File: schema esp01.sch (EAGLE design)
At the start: 8 parts

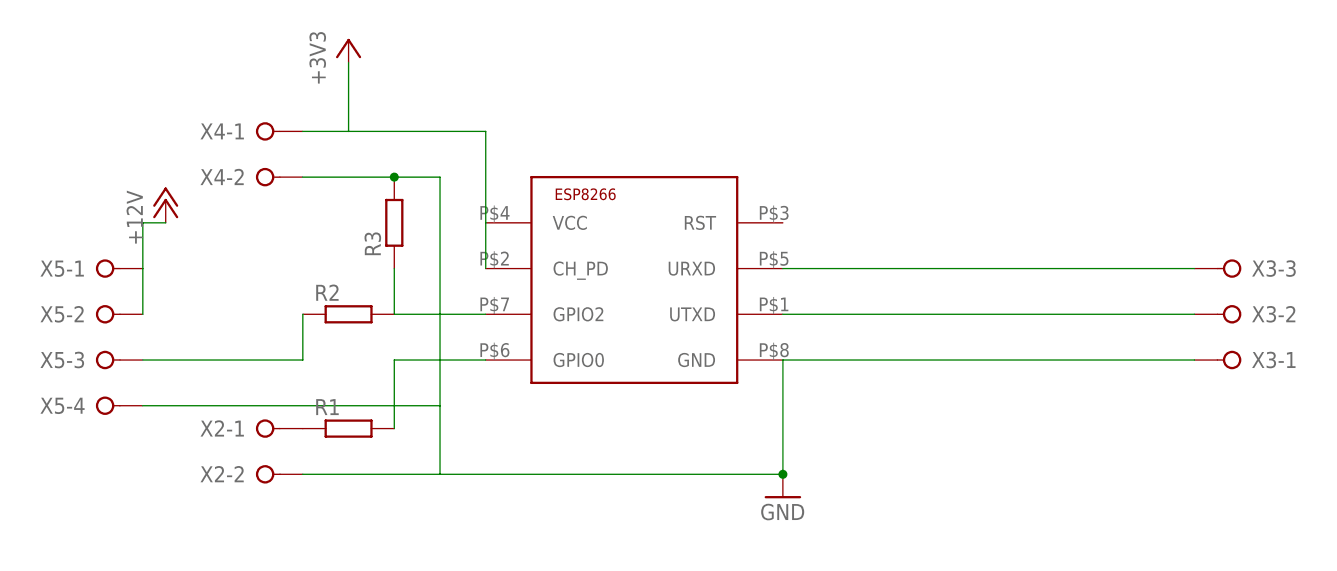
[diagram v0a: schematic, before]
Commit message: +
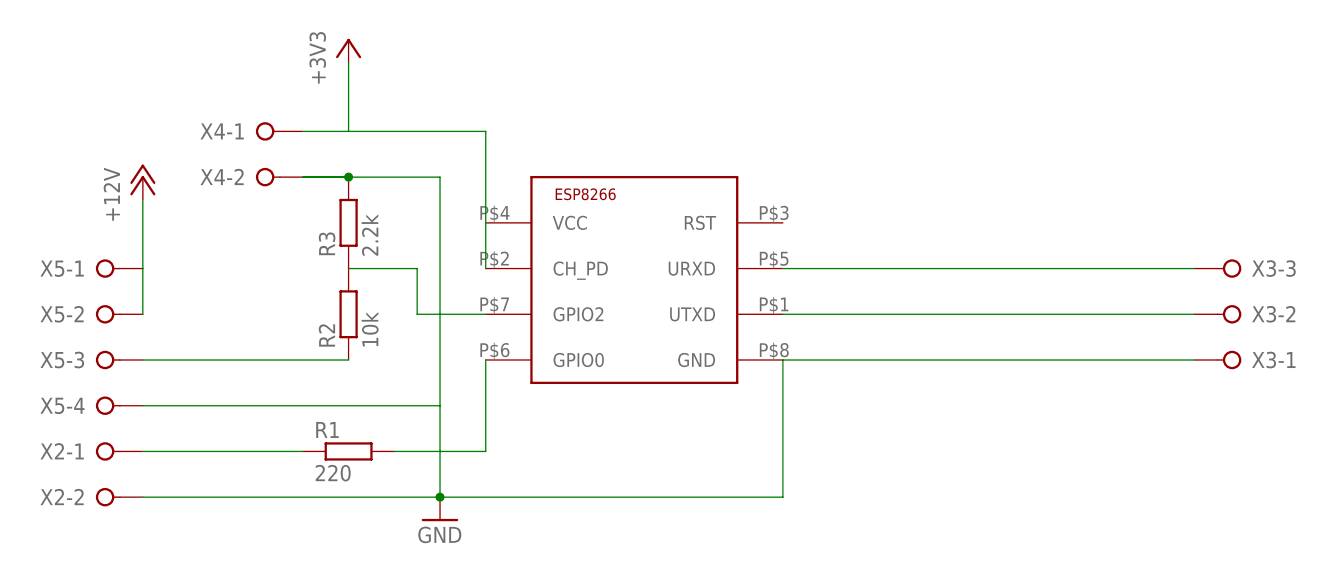
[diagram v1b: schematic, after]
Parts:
- R1: value (none) -> 220
- R2: value (none) -> 10k
- R3: value (none) -> 2.2k
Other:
- moved on the sheet: R1, R2, R3, X2-1, X2-2
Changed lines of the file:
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@@
 <part name="X2" library="con-wago-508" deviceset="W237-02P" device=""/>
 <part name="X3" library="con-wago-508" deviceset="W237-3E" device=""/>
-<part name="R1" library="rcl" deviceset="R-EU_" device="0204/7"/>
+<part name="R1" library="rcl" deviceset="R-EU_" device="0204/7" value="220"/>
 <part name="X4" library="con-wago-508" deviceset="W237-02P" device=""/>
 <part name="+3V1" library="supply1" deviceset="+3V3" device=""/>
-<part name="R2" library="rcl" deviceset="R-EU_" device="0204/7"/>
-<part name="R3" library="rcl" deviceset="R-EU_" device="0204/7"/>
+<part name="R2" library="rcl" deviceset="R-EU_" device="0204/7" value="10k"/>
+<part name="R3" library="rcl" deviceset="R-EU_" device="0204/7" value="2.2k"/>
 <part name="X5" library="con-wago-508" deviceset="W237-04P" device=""/>
 <part name="P+1" library="supply1" deviceset="+12V" device=""/>
@@
 <instances>
 <instance part="U$1" gate="G$1" x="12.7" y="68.58"/>
-<instance part="X2" gate="-1" x="-12.7" y="60.96"/>
-<instance part="X2" gate="-2" x="-12.7" y="55.88"/>
+<instance part="X2" gate="-1" x="-30.48" y="58.42"/>
+<instance part="X2" gate="-2" x="-30.48" y="53.34"/>
 <instance part="X3" gate="-1" x="96.52" y="68.58" rot="R180"/>
 <instance part="X3" gate="-2" x="96.52" y="73.66" rot="R180"/>
 <instance part="X3" gate="-3" x="96.52" y="78.74" rot="R180"/>
-<instance part="R1" gate="G$1" x="-2.54" y="60.96"/>
+<instance part="R1" gate="G$1" x="-2.54" y="58.42"/>
 <instance part="X4" gate="-1" x="-12.7" y="93.98"/>
 <instance part="X4" gate="-2" x="-12.7" y="88.9"/>
 <instance part="+3V1" gate="G$1" x="-2.54" y="104.14"/>
-<instance part="R2" gate="G$1" x="-2.54" y="73.66"/>
-<instance part="R3" gate="G$1" x="2.54" y="83.82" rot="R90"/>
+<instance part="R2" gate="G$1" x="-2.54" y="73.66" rot="R90"/>
+<instance part="R3" gate="G$1" x="-2.54" y="83.82" rot="R90"/>
 <instance part="X5" gate="-1" x="-30.48" y="78.74"/>
 <instance part="X5" gate="-2" x="-30.48" y="73.66"/>
 <instance part="X5" gate="-3" x="-30.48" y="68.58"/>
 <instance part="X5" gate="-4" x="-30.48" y="63.5"/>
-<instance part="P+1" gate="1" x="-22.86" y="86.36"/>
-<instance part="GND1" gate="1" x="45.72" y="53.34"/>
+<instance part="P+1" gate="1" x="-25.4" y="88.9"/>
+<instance part="GND1" gate="1" x="7.62" y="50.8"/>
 </instances>
 <busses>
@@
 <pinref part="X2" gate="-1" pin="KL"/>
 <pinref part="R1" gate="G$1" pin="1"/>
+<wire x1="-25.4" y1="58.42" x2="-7.62" y2="58.42" width="0.1524" layer="91"/>
 </segment>
 </net>
@@
 <segment>
 <pinref part="R1" gate="G$1" pin="2"/>
-<wire x1="2.54" y1="60.96" x2="2.54" y2="68.58" width="0.1524" layer="91"/>
+<wire x1="2.54" y1="58.42" x2="12.7" y2="58.42" width="0.1524" layer="91"/>
 <pinref part="U$1" gate="G$1" pin="GPIO0"/>
-<wire x1="2.54" y1="68.58" x2="12.7" y2="68.58" width="0.1524" layer="91"/>
+<wire x1="12.7" y1="58.42" x2="12.7" y2="68.58" width="0.1524" layer="91"/>
 </segment>
 </net>
@@
 <pinref part="R2" gate="G$1" pin="2"/>
 <pinref part="R3" gate="G$1" pin="1"/>
-<wire x1="2.54" y1="73.66" x2="2.54" y2="78.74" width="0.1524" layer="91"/>
 <pinref part="U$1" gate="G$1" pin="GPIO2"/>
-<wire x1="12.7" y1="73.66" x2="2.54" y2="73.66" width="0.1524" layer="91"/>
+<wire x1="12.7" y1="73.66" x2="5.08" y2="73.66" width="0.1524" layer="91"/>
+<wire x1="5.08" y1="73.66" x2="5.08" y2="78.74" width="0.1524" layer="91"/>
+<wire x1="5.08" y1="78.74" x2="-2.54" y2="78.74" width="0.1524" layer="91"/>
 </segment>
 </net>
@@
 <pinref part="P+1" gate="1" pin="+12V"/>
 <pinref part="X5" gate="-1" pin="KL"/>
-<wire x1="-22.86" y1="83.82" x2="-25.4" y2="83.82" width="0.1524" layer="91"/>
-<wire x1="-25.4" y1="83.82" x2="-25.4" y2="78.74" width="0.1524" layer="91"/>
+<wire x1="-25.4" y1="86.36" x2="-25.4" y2="78.74" width="0.1524" layer="91"/>
 <pinref part="X5" gate="-2" pin="KL"/>
 <wire x1="-25.4" y1="78.74" x2="-25.4" y2="73.66" width="0.1524" layer="91"/>
@@
 <pinref part="X2" gate="-2" pin="KL"/>
 <pinref part="U$1" gate="G$1" pin="GND"/>
-<wire x1="-7.62" y1="55.88" x2="7.62" y2="55.88" width="0.1524" layer="91"/>
-<wire x1="7.62" y1="55.88" x2="45.72" y2="55.88" width="0.1524" layer="91"/>
-<wire x1="45.72" y1="55.88" x2="45.72" y2="68.58" width="0.1524" layer="91"/>
+<wire x1="-25.4" y1="53.34" x2="7.62" y2="53.34" width="0.1524" layer="91"/>
+<wire x1="7.62" y1="53.34" x2="45.72" y2="53.34" width="0.1524" layer="91"/>
+<wire x1="45.72" y1="53.34" x2="45.72" y2="68.58" width="0.1524" layer="91"/>
 <pinref part="X4" gate="-2" pin="KL"/>
-<wire x1="-7.62" y1="88.9" x2="2.54" y2="88.9" width="0.1524" layer="91"/>
-<wire x1="2.54" y1="88.9" x2="7.62" y2="88.9" width="0.1524" layer="91"/>
+<wire x1="-2.54" y1="88.9" x2="-7.62" y2="88.9" width="0.1524" layer="91"/>
+<wire x1="-7.62" y1="88.9" x2="7.62" y2="88.9" width="0.1524" layer="91"/>
 <wire x1="7.62" y1="88.9" x2="7.62" y2="63.5" width="0.1524" layer="91"/>
-<wire x1="7.62" y1="63.5" x2="7.62" y2="55.88" width="0.1524" layer="91"/>
+<wire x1="7.62" y1="63.5" x2="7.62" y2="53.34" width="0.1524" layer="91"/>
 <wire x1="45.72" y1="68.58" x2="91.44" y2="68.58" width="0.1524" layer="91"/>
 <pinref part="X3" gate="-1" pin="KL"/>
 <pinref part="R3" gate="G$1" pin="2"/>
-<junction x="2.54" y="88.9"/>
+<junction x="-2.54" y="88.9"/>
 <pinref part="X5" gate="-4" pin="KL"/>
 <wire x1="-25.4" y1="63.5" x2="7.62" y2="63.5" width="0.1524" layer="91"/>
 <pinref part="GND1" gate="1" pin="GND"/>
-<junction x="45.72" y="55.88"/>
+<junction x="7.62" y="53.34"/>
 </segment>
 </net>
@@
 <pinref part="X5" gate="-3" pin="KL"/>
 <pinref part="R2" gate="G$1" pin="1"/>
-<wire x1="-25.4" y1="68.58" x2="-7.62" y2="68.58" width="0.1524" layer="91"/>
-<wire x1="-7.62" y1="68.58" x2="-7.62" y2="73.66" width="0.1524" layer="91"/>
+<wire x1="-25.4" y1="68.58" x2="-2.54" y2="68.58" width="0.1524" layer="91"/>
 </segment>
 </net>
